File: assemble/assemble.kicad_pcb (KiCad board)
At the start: 2 copper layers, 272.2 x 100.7 mm, 122 parts, among them J1 Conn_02x04_Odd_Even, SW1 SW_Push, SW10 SW_Push, SW11 SW_Push, SW12 SW_Push, SW13 SW_Push, SW14 SW_Push, SW15 SW_Push, SW16 SW_Push, SW17 SW_Push, SW18 SW_Push, SW19 SW_Push, SW2 SW_Push, SW20 SW_Push, SW21 SW_Push, SW22 SW_Push, SW23 SW_Push, SW24 SW_Push, SW25 SW_Push, SW26 SW_Push, SW27 SW_Push, SW28 SW_Push, SW29 SW_Push, SW3 SW_Push, SW30 SW_Push, SW31 SW_Push, SW32 SW_Push, SW33 SW_Push, SW34 SW_Push, SW35 SW_Push, SW36 SW_Push, SW37 SW_Push, SW38 SW_Push, SW39 SW_Push, SW4 SW_Push, SW40 SW_Push, SW41 SW_Push, SW42 SW_Push, SW43 SW_SPDT, SW44 SW_SPDT, SW45 RotaryEncoder_Switch, SW5 SW_Push, SW6 SW_Push, SW7 SW_Push, SW8 SW_Push, SW9 SW_Push, U1 XIAO-nRF52840-SMD, U2 XIAO-nRF52840-SMD

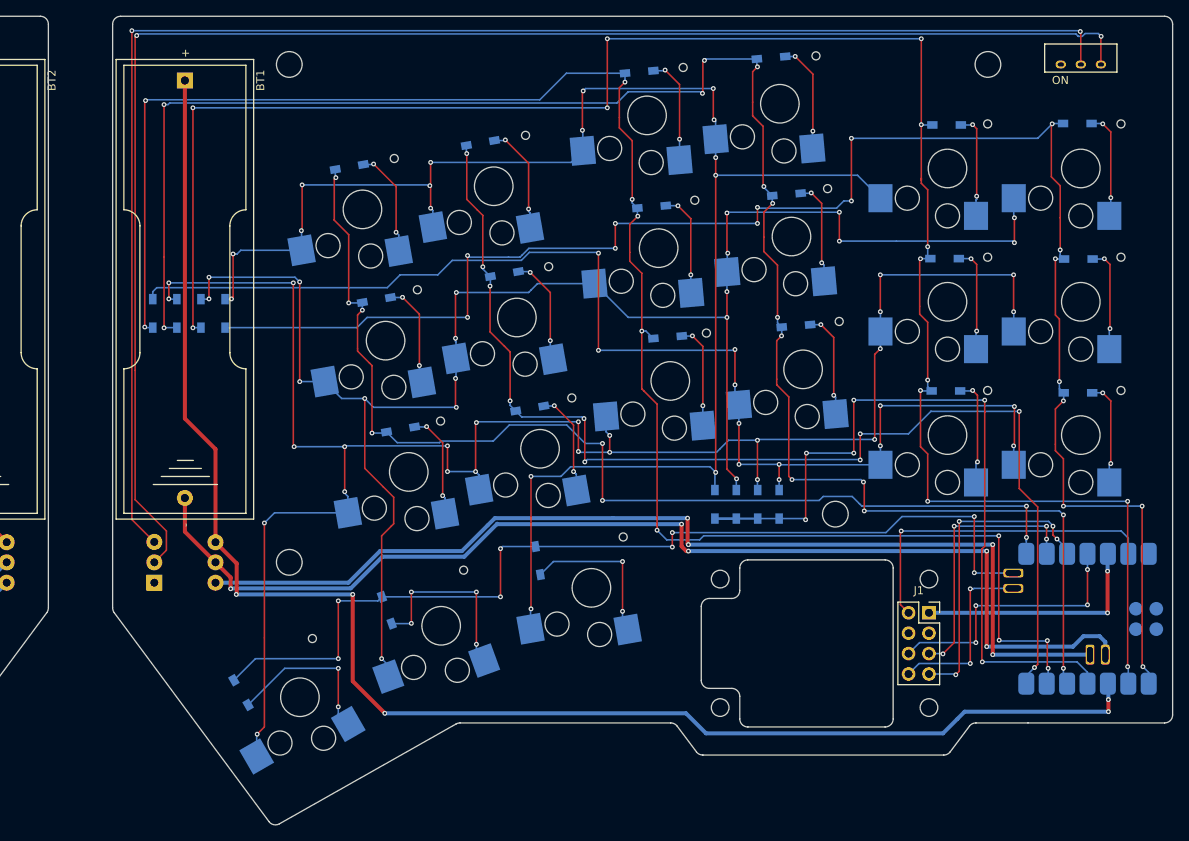
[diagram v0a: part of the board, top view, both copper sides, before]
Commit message: fix: case problems
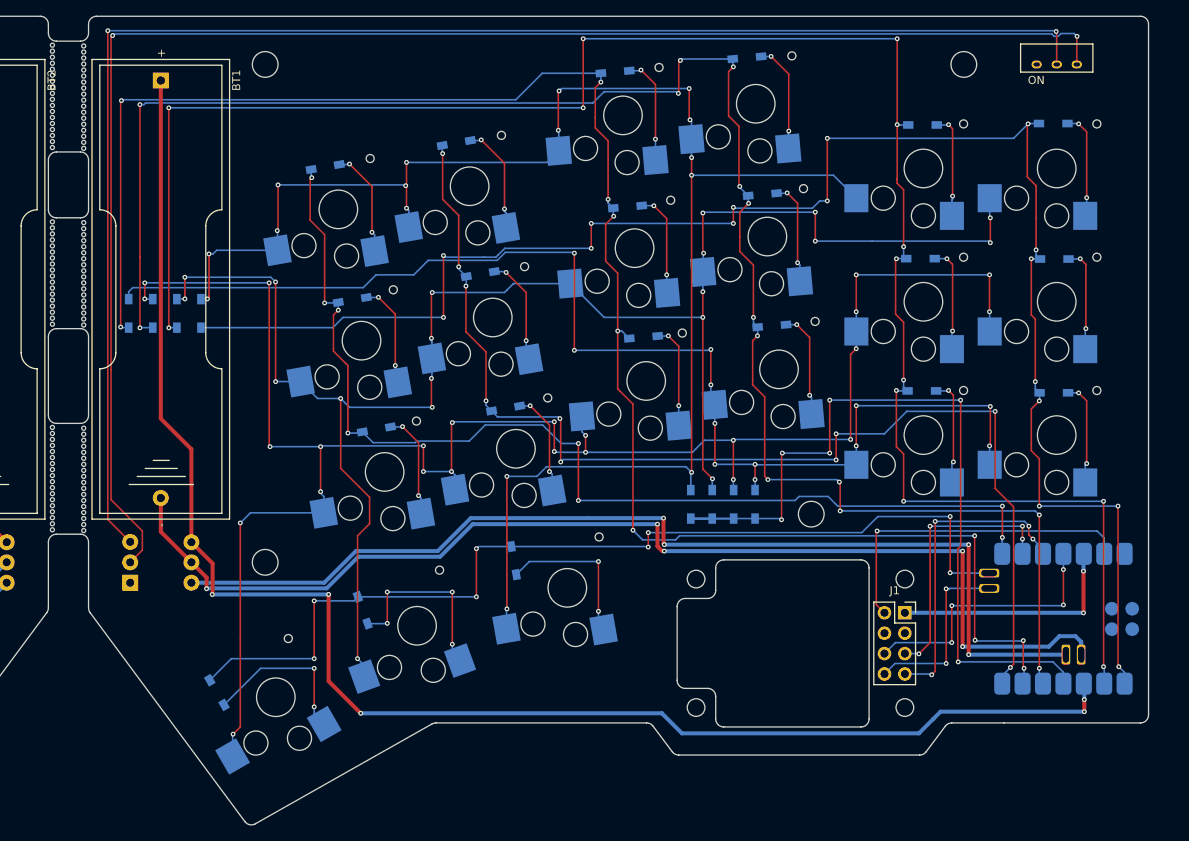
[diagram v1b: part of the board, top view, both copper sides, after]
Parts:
- added Ref**: Val**, kbd_Hole:Mouse_Bite_Hole, F.Cu at (151.5, 69.5)
- added Ref**: Val**, kbd_Hole:Mouse_Bite_Hole, F.Cu at (155.4, 47.6)
- added Ref**: Val**, kbd_Hole:Mouse_Bite_Hole, F.Cu at (155.4, 43.1)
- added Ref**: Val**, kbd_Hole:Mouse_Bite_Hole, F.Cu at (155.4, 65.1)
- added Ref**: Val**, kbd_Hole:Mouse_Bite_Hole, F.Cu at (151.5, 60.5)
- added Ref**: Val**, kbd_Hole:Mouse_Bite_Hole, F.Cu at (155.4, 86.2)
- added Ref**: Val**, kbd_Hole:Mouse_Bite_Hole, F.Cu at (151.5, 43.0)
- added Ref**: Val**, kbd_Hole:Mouse_Bite_Hole, F.Cu at (151.5, 47.5)
- added Ref**: Val**, kbd_Hole:Mouse_Bite_Hole, F.Cu at (151.5, 95.1)
- added Ref**: Val**, kbd_Hole:Mouse_Bite_Hole, F.Cu at (155.4, 90.7)
- added Ref**: Val**, kbd_Hole:Mouse_Bite_Hole, F.Cu at (155.4, 60.6)
- added Ref**: Val**, kbd_Hole:Mouse_Bite_Hole, F.Cu at (155.4, 38.6)
- added Ref**: Val**, kbd_Hole:Mouse_Bite_Hole, F.Cu at (155.4, 69.6)
- added Ref**: Val**, kbd_Hole:Mouse_Bite_Hole, F.Cu at (151.5, 86.1)
- added Ref**: Val**, kbd_Hole:Mouse_Bite_Hole, F.Cu at (155.4, 95.2)
- added Ref**: Val**, kbd_Hole:Mouse_Bite_Hole, F.Cu at (151.5, 38.5)
- added Ref**: Val**, kbd_Hole:Mouse_Bite_Hole, F.Cu at (151.5, 90.6)
- added Ref**: Val**, kbd_Hole:Mouse_Bite_Hole, F.Cu at (151.5, 65.0)
- moved AE-XCL102D333CR-G1 3.00 mm to (165.0, 101.0)
- moved BT1 3.00 mm to (165.0, 41.0)
- moved D10 3.00 mm to (170.0, 70.0)
- moved D14 3.00 mm to (276.1, 46.4)
- moved D15 3.00 mm to (276.3, 63.2)
- moved D16 3.00 mm to (276.2, 79.9)
- moved D18 3.00 mm to (167.0, 70.0)
- moved D22 3.00 mm to (259.9, 46.5)
- moved D23 3.00 mm to (259.6, 63.2)
- moved D24 3.00 mm to (259.8, 79.7)
- moved D26 3.00 mm to (164.0, 70.0)
- moved D30 3.00 mm to (238.0, 38.2)
- moved D31 3.00 mm to (239.9, 55.2)
- moved D32 3.00 mm to (241.1, 71.6)
- moved D34 3.00 mm to (161.0, 70.0)
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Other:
- board size 272.2 x 100.7 mm -> 269.2 x 100.7 mm
